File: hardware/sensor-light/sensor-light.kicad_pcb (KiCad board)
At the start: 2 copper layers, 17 parts, among them J1 Power IN 12V, J2 PIR Sensor 2, J3 PIR Sensor 1, J4 PROG Header, J5 Light Sensor, J6 PWM Power OUT 12V, Q1 IRLML2502, SW1 Manual ON/OFF, U1 Reg 3.3V, U2 MSP430G2553IN20

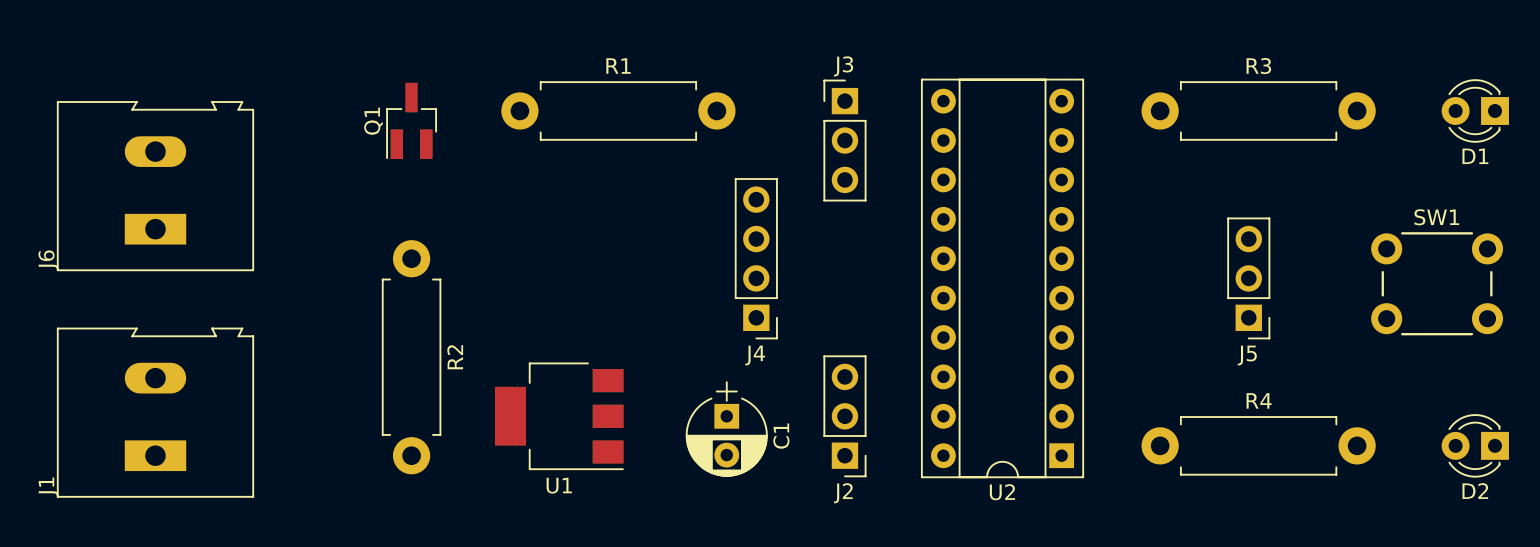
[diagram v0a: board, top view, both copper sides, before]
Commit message: some attempt of pcb routing
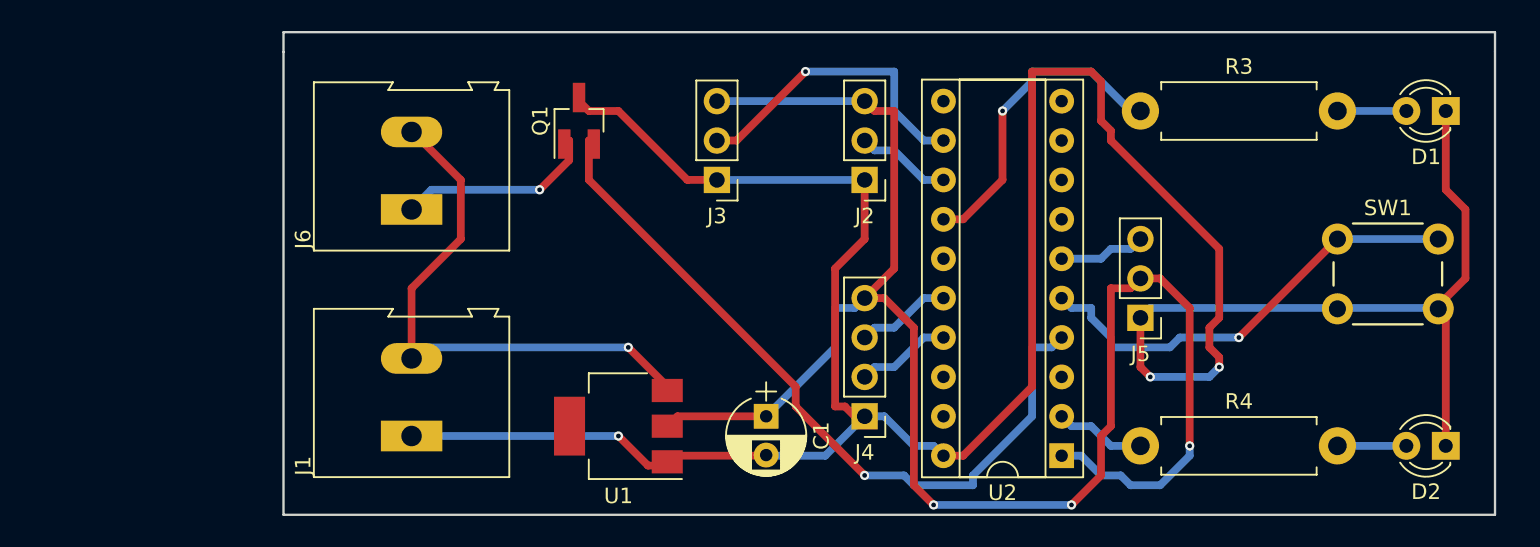
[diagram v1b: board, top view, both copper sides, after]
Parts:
- removed R1: 27 Ohm, Resistors_THT:R_Axial_DIN0411_L9.9mm_D3.6mm_P12.70mm_Horizontal
- removed R2: 100 KOhm, Resistors_THT:R_Axial_DIN0411_L9.9mm_D3.6mm_P12.70mm_Horizontal
- J2: value PIR Sensor 2 -> PIR 2
- J3: value PIR Sensor 1 -> PIR 1
- J6: value PWM Power OUT 12V -> Power OUT 12V
- moved J2 17.8 mm to (153.7, 116.2)
- moved J1 16.6 mm to (124.5, 132.7)
- moved J6 16.6 mm to (124.5, 118.1)
- moved Q1 10.8 mm to (135.3, 112.4)
- moved J3 9.69 mm to (144.1, 116.2), turned to 180 degrees
- moved J4 9.44 mm to (153.7, 131.4)
- moved J5 6.99 mm to (171.4, 125.1)
- moved U1 3.86 mm to (137.8, 132.1)
- moved SW1 3.24 mm to (184.2, 120.0)
- moved D1 3.18 mm to (191.1, 111.8)
- moved D2 3.18 mm to (191.1, 133.3)
- moved C1 2.54 mm to (147.3, 131.4)
- moved R3 1.27 mm to (171.4, 111.8)
- moved R4 1.27 mm to (171.4, 133.3)
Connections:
- J6 pad 1: Net-(J1-Pad2) -> Net-(J6-Pad1)
- J6 pad 2: Net-(J6-Pad2) -> Net-(J1-Pad2)
- Q1 pad 1: Net-(J6-Pad2) -> Net-(J6-Pad1)
- U2 pad 4: Net-(R1-Pad2) -> Net-(Q1-Pad2)
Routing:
- net Net-(C1-Pad2): track 0.00 -> 182.9 mm, vias 0 -> 3
- net Net-(C1-Pad1): track 0.00 -> 107.5 mm, vias 0 -> 3
- net Net-(Q1-Pad2): track 0.00 -> 49.2 mm, vias 0 -> 1
- net Net-(J1-Pad2): track 0.00 -> 35.5 mm, vias 0 -> 1
- net Net-(SW1-Pad1): track 0.00 -> 29.2 mm, vias 0 -> 1
- net Net-(R3-Pad1): track 0.00 -> 20.7 mm, vias 0 -> 1
- net Net-(J3-Pad2): track 0.00 -> 19.8 mm, vias 0 -> 1
- net Net-(J6-Pad1): track 0.00 -> 13.1 mm, vias 0 -> 1
- net Net-(J4-Pad2): track 0.00 -> 6.13 mm
- net Net-(J4-Pad3): track 0.00 -> 6.13 mm
- net Net-(J2-Pad2): track 0.00 -> 6.13 mm
- net Net-(R4-Pad1): track 0.00 -> 5.87 mm
- net Net-(J5-Pad3): track 0.00 -> 5.61 mm
- net Net-(D2-Pad2): track 0.00 -> 4.44 mm
- net Net-(D1-Pad2): track 0.00 -> 4.44 mm
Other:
- board outline added: 78.1 x 31.1 mm
- net class Default: clearance 0.2 -> 0.5; trace_width 0.25 -> 0.5
- rule trace_clearance: 0.2 -> 0.5
